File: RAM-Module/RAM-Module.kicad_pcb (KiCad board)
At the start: 2 copper layers, 21 parts, among them J15 RAM Module

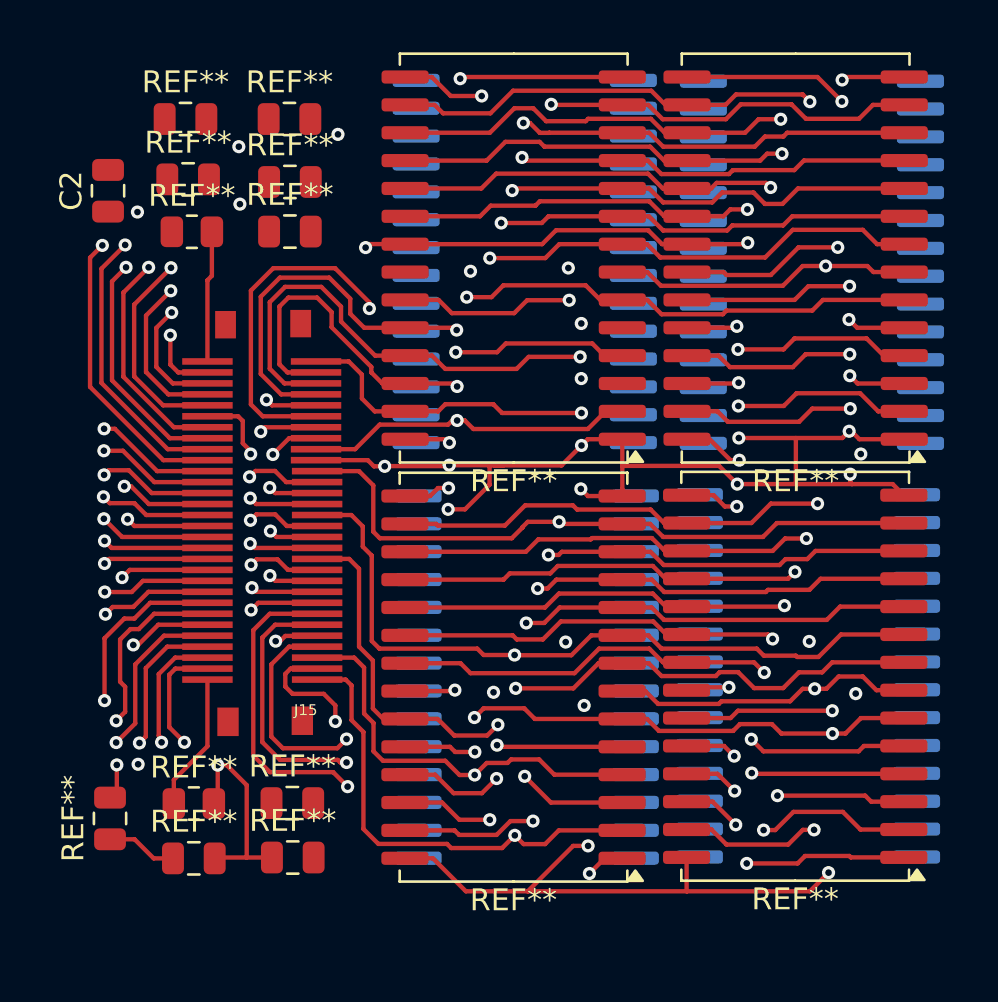
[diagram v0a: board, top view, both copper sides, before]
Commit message: Add files via upload
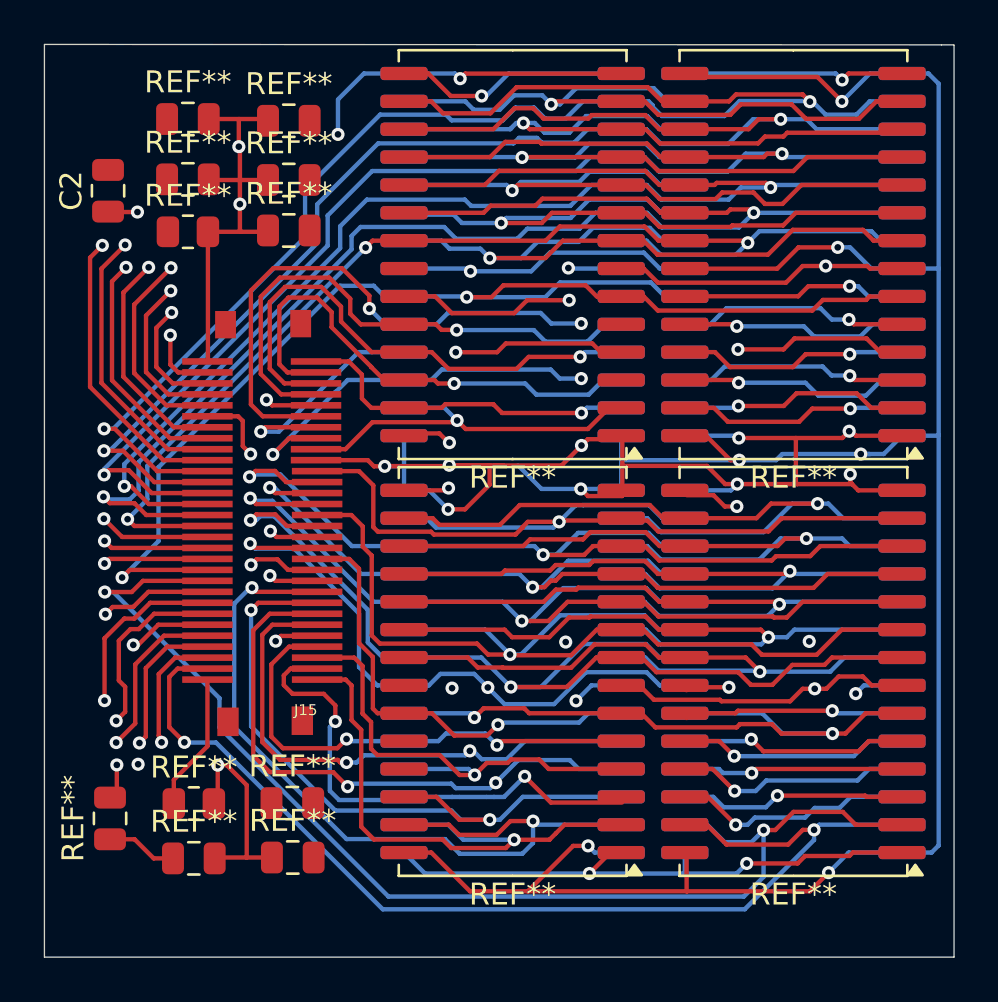
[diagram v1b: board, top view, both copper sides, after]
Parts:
- moved REF** 0.91 mm to (143.2, 88.0)
- moved REF** 0.69 mm to (143.2, 107.0)
- moved REF** 0.69 mm to (130.4, 107.0)
- moved REF** 0.63 mm to (130.4, 88.0)
- moved REF** 0.26 mm to (130.4, 107.0)
- moved REF** 0.23 mm to (143.2, 107.0)
- moved REF** 0.19 mm to (143.2, 88.0)
- moved REF** 0.18 mm to (115.6, 87.0)
- moved REF** 0.17 mm to (130.4, 88.0)
- moved REF** 0.11 mm to (115.6, 81.8)
- moved REF** 0.10 mm to (120.2, 84.6)
- moved REF** 0.09 mm to (120.2, 81.9)
- moved REF** 0.07 mm to (120.2, 86.9)
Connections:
- J15 pad 1: (no net) -> J1_1
- J15 pad 11: (no net) -> J1_11
- J15 pad 12: (no net) -> J1_12
- J15 pad 13: (no net) -> J1_13
- J15 pad 14: (no net) -> J1_14
- J15 pad 15: (no net) -> J1_15
- J15 pad 16: (no net) -> J1_16
- J15 pad 17: (no net) -> J1_17
- J15 pad 18: (no net) -> J1_18
- J15 pad 19: (no net) -> J1_19
- J15 pad 2: (no net) -> J1_2
- J15 pad 20: (no net) -> J1_20
- J15 pad 21: (no net) -> J1_21
- J15 pad 22: (no net) -> J1_22
- J15 pad 23: (no net) -> J1_23
- J15 pad 24: (no net) -> J1_24
- J15 pad 25: (no net) -> J1_25
- J15 pad 26: (no net) -> J1_26
- J15 pad 27: (no net) -> J1_27
- J15 pad 28: (no net) -> J1_28
- J15 pad 29: (no net) -> J1_29
- J15 pad 3: (no net) -> J1_3
- J15 pad 30: (no net) -> J1_30
- J15 pad 31: (no net) -> J1_31
- J15 pad 32: (no net) -> J1_32
- J15 pad 33: (no net) -> J1_33
- J15 pad 34: (no net) -> J1_34
- J15 pad 35: (no net) -> J1_35
- J15 pad 36: (no net) -> J1_36
- J15 pad 37: (no net) -> J1_37
- J15 pad 38: (no net) -> J1_38
- J15 pad 39: (no net) -> J1_39
- J15 pad 4: (no net) -> J1_4
- J15 pad 40: (no net) -> J1_40
- J15 pad 41: (no net) -> J1_41
- J15 pad 42: (no net) -> J1_42
- J15 pad 43: (no net) -> J1_43
- J15 pad 44: (no net) -> J1_44
- J15 pad 45: (no net) -> J1_45
- J15 pad 46: (no net) -> J1_46
- J15 pad 47: (no net) -> J1_47
- J15 pad 48: (no net) -> J1_48
- J15 pad 49: (no net) -> J1_49
- J15 pad 5: (no net) -> J1_5
- J15 pad 50: (no net) -> J1_50
- J15 pad 51: (no net) -> J1_51
- J15 pad 52: (no net) -> J1_52
- J15 pad 53: (no net) -> J1_53
- J15 pad 54: (no net) -> J1_54
- J15 pad 55: (no net) -> J1_55
- J15 pad 56: (no net) -> J1_56
- J15 pad 57: (no net) -> J1_57
- J15 pad 58: (no net) -> J1_58
- J15 pad 59: (no net) -> J1_59
- J15 pad 6: (no net) -> J1_6
- J15 pad 60: (no net) -> J1_60
- J15 pad 7: (no net) -> J1_7
- J15 pad 8: (no net) -> J1_8
- J15 pad 9: (no net) -> J1_9
- REF** pad 2: (no net) -> J1_60 (x3)
- REF** pad 16: (no net) -> J1_50 (x4)
- REF** pad 17: (no net) -> J1_49 (x4)
- REF** pad 18: (no net) -> J1_48 (x4)
- REF** pad 19: (no net) -> J1_47 (x4)
- REF** pad 20: (no net) -> J1_46 (x4)
- REF** pad 21: (no net) -> J1_45 (x4)
- REF** pad 6: (no net) -> J1_41 (x4)
- REF** pad 1: (no net) -> J1_60 (x3)
- REF** pad 10: (no net) -> J1_14 (x4)
- REF** pad 11: (no net) -> J1_13 (x4)
- REF** pad 12: (no net) -> J1_12 (x4)
- REF** pad 13: (no net) -> J1_11 (x4)
- REF** pad 2: (no net) -> J1_30 (x2)
- REF** pad 23: (no net) -> J1_19 (x2)
- REF** pad 26: (no net) -> J1_23 (x2)
- REF** pad 27: (no net) -> J1_22 (x2)
- REF** pad 3: (no net) -> J1_29 (x2)
- REF** pad 4: (no net) -> J1_28 (x2)
- REF** pad 5: (no net) -> J1_27 (x2)
- REF** pad 8: (no net) -> J1_16 (x4)
- REF** pad 9: (no net) -> J1_15 (x4)
- REF** pad 1: (no net) -> J1_10 (x2)
- REF** pad 28: (no net) -> J1_10 (x2)
- REF** pad 14: (no net) -> J1_10 (x2)
- REF** pad 15: (no net) -> J1_10
- REF** pad 24: (no net) -> J1_25
- REF** pad 25: (no net) -> J1_24
- REF** pad 7: (no net) -> J1_18 (x2)
- REF** pad 2: (no net) -> J1_9 (x2)
- REF** pad 24: (no net) -> J1_4 (x2)
- REF** pad 25: (no net) -> J1_3 (x2)
- REF** pad 26: (no net) -> J1_2 (x2)
- REF** pad 27: (no net) -> J1_1 (x2)
- REF** pad 3: (no net) -> J1_8
- REF** pad 4: (no net) -> J1_7
- REF** pad 5: (no net) -> J1_6
- REF** pad 2: (no net) -> J1_40
- REF** pad 27: (no net) -> J1_32
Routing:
- net (no net): track 1192.3 -> 728.7 mm, vias 143 -> 55
- net J1_10: track 46.7 -> 177.6 mm, vias 9 -> 15
- net J1_50: track 0.00 -> 70.8 mm, vias 0 -> 2
- net J1_49: track 0.00 -> 68.2 mm, vias 0 -> 2
- net J1_48: track 0.00 -> 67.1 mm, vias 0 -> 2
- net J1_46: track 0.00 -> 65.7 mm, vias 0 -> 2
- net J1_47: track 0.00 -> 64.6 mm, vias 0 -> 2
- net J1_41: track 0.00 -> 58.7 mm, vias 0 -> 2
- net J1_40: track 0.00 -> 55.0 mm, vias 0 -> 2
- net J1_45: track 0.00 -> 52.4 mm, vias 0 -> 3
- net J1_32: track 0.00 -> 49.4 mm, vias 0 -> 2
- net J1_16: track 0.00 -> 47.8 mm, vias 0 -> 2
- net J1_15: track 0.00 -> 47.7 mm, vias 0 -> 1
- net J1_14: track 0.00 -> 44.5 mm, vias 0 -> 2
- net J1_11: track 0.00 -> 43.6 mm, vias 0 -> 1
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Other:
- board outline added: 41.5 x 41.6 mm
